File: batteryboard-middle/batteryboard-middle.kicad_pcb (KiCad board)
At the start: 2 copper layers, 45.6 x 45.6 mm, 15 parts, among them J1 FLE-107-01-X-DV-A, J2 FTS-107-01-X-DV-A, J3 Battery Pads, J4 Battery Pads

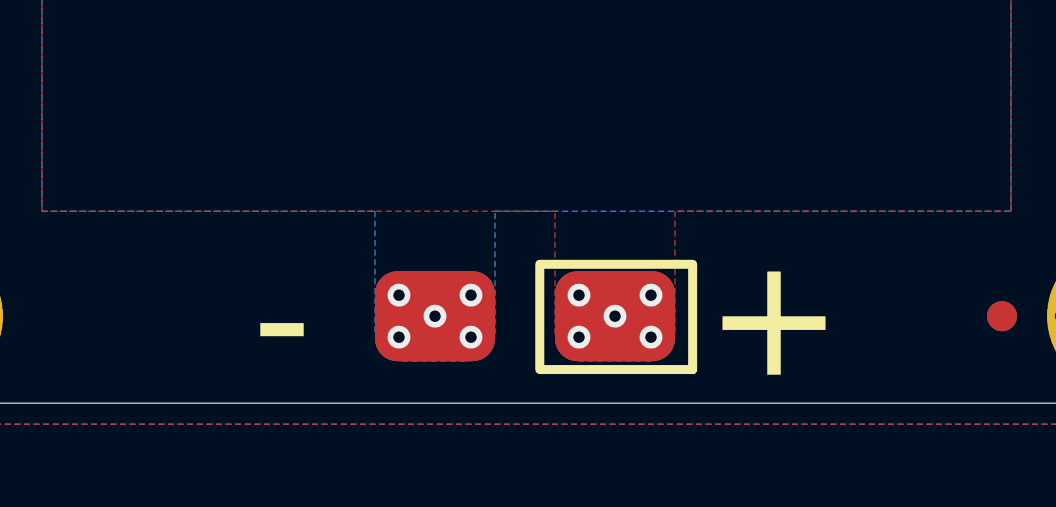
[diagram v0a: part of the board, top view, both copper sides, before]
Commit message: Updated BOMs and STEP files
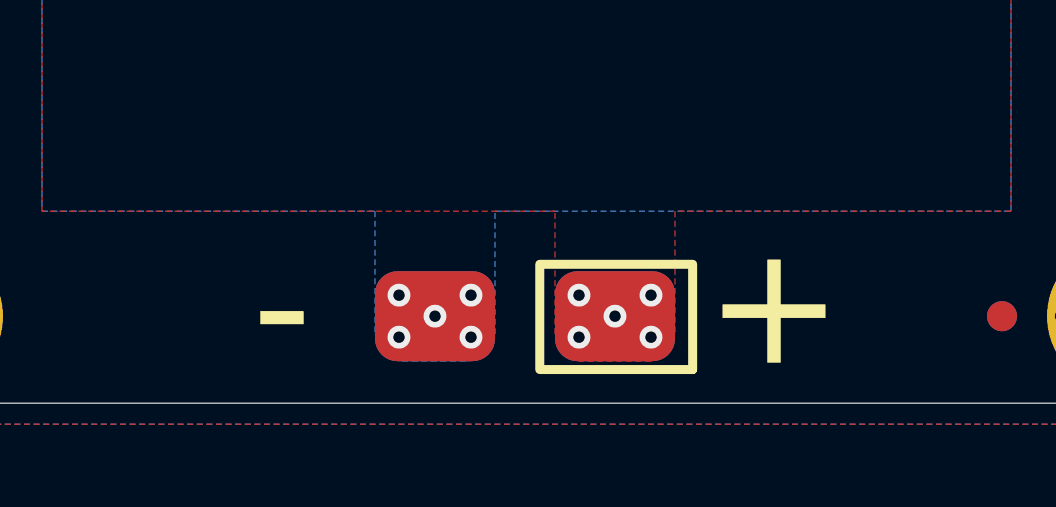
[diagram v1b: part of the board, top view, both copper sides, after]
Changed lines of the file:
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@@
     (property "Sheetfile" "batteryboard-middle.kicad_sch")
     (property "Sheetname" "")
+    (property "exclude_from_bom" "")
     (property "ki_description" "Mounting Hole with connection")
     (property "ki_keywords" "mounting hole")
@@
     (property "Sheetfile" "batteryboard-middle.kicad_sch")
     (property "Sheetname" "")
+    (property "exclude_from_bom" "")
     (property "ki_description" "Mounting Hole with connection")
     (property "ki_keywords" "mounting hole")
@@
     (property "Sheetfile" "batteryboard-middle.kicad_sch")
     (property "Sheetname" "")
+    (property "exclude_from_bom" "")
     (property "ki_description" "Generic connector, single row, 01x02, script generated (kicad-library-utils/schlib/autogen/connector/)")
     (property "ki_keywords" "connector")
-    (attr smd)
+    (attr smd exclude_from_bom)
     (fp_text reference "J3" (at -7.111997 -0.000005 180 unlocked) (layer "F.SilkS") hide
         (effects (font (size 1 1) (thickness 0.15)))
@@
     (descr "Circular Fiducial, 1mm bare copper, 2mm soldermask opening (Level A)")
     (tags "fiducial")
-    (attr smd)
+    (attr smd exclude_from_bom)
     (fp_text reference "REF**" (at 0 -2) (layer "F.SilkS") hide
         (effects (font (size 1 1) (thickness 0.15)))
@@
   (footprint "custom-footprints:pycubed_mini_half" (layer "F.Cu")
     (at 103.9 45)
-    (attr through_hole)
+    (attr through_hole exclude_from_bom)
     (fp_text reference "Ref**" (at 0 0) (layer "F.SilkS") hide
         (effects (font (size 1.27 1.27) (thickness 0.15)))
@@
     (property "Sheetfile" "batteryboard-middle.kicad_sch")
     (property "Sheetname" "")
+    (property "exclude_from_bom" "")
     (property "ki_description" "Mounting Hole with connection")
     (property "ki_keywords" "mounting hole")
@@
     (property "Sheetfile" "batteryboard-middle.kicad_sch")
     (property "Sheetname" "")
+    (property "exclude_from_bom" "")
     (property "ki_description" "Mounting Hole with connection")
     (property "ki_keywords" "mounting hole")
@@
     (descr "Circular Fiducial, 1mm bare copper, 2mm soldermask opening (Level A)")
     (tags "fiducial")
-    (attr smd)
+    (attr smd exclude_from_bom)
     (fp_text reference "REF**" (at 0 -2) (layer "F.SilkS") hide
         (effects (font (size 1 1) (thickness 0.15)))
@@
     (descr "Circular Fiducial, 1mm bare copper, 2mm soldermask opening (Level A)")
     (tags "fiducial")
-    (attr smd)
+    (attr smd exclude_from_bom)
     (fp_text reference "REF**" (at 0 -2) (layer "F.SilkS") hide
         (effects (font (size 1 1) (thickness 0.15)))
@@
     (property "Sheetfile" "batteryboard-middle.kicad_sch")
     (property "Sheetname" "")
+    (property "exclude_from_bom" "")
     (property "ki_description" "Generic connector, single row, 01x02, script generated (kicad-library-utils/schlib/autogen/connector/)")
     (property "ki_keywords" "connector")
-    (attr smd)
+    (attr smd exclude_from_bom)
     (fp_text reference "J4" (at -7.112 0 180 unlocked) (layer "B.SilkS") hide
         (effects (font (size 1 1) (thickness 0.15)) (justify mirror))
@@
     (descr "Circular Fiducial, 1mm bare copper, 2mm soldermask opening (Level A)")
     (tags "fiducial")
-    (attr smd)
+    (attr smd exclude_from_bom)
     (fp_text reference "REF**" (at 0 2) (layer "B.SilkS") hide
         (effects (font (size 1 1) (thickness 0.15)) (justify mirror))
@@
     (descr "Circular Fiducial, 1mm bare copper, 2mm soldermask opening (Level A)")
     (tags "fiducial")
-    (attr smd)
+    (attr smd exclude_from_bom)
     (fp_text reference "REF**" (at 0 2) (layer "B.SilkS") hide
         (effects (font (size 1 1) (thickness 0.15)) (justify mirror))
@@
     (descr "Circular Fiducial, 1mm bare copper, 2mm soldermask opening (Level A)")
     (tags "fiducial")
-    (attr smd)
+    (attr smd exclude_from_bom)
     (fp_text reference "REF**" (at 0 2) (layer "B.SilkS") hide
         (effects (font (size 1 1) (thickness 0.15)) (justify mirror))
@@
   (gr_line (start 123.1 88.3) (end 83.3 88.3)
     (stroke (width 0.0254) (type solid)) (layer "Edge.Cuts"))
-  (gr_text "+" (at 111.5 85.5) (layer "B.SilkS")
+  (gr_text "+" (at 111.5 85.1) (layer "B.SilkS")
     (effects (font (size 4 4) (thickness 0.7)) (justify mirror))
   )
-  (gr_text "-" (at 95.1 85.5) (layer "B.SilkS")
+  (gr_text "-" (at 95.1 85.1) (layer "B.SilkS")
     (effects (font (size 4 4) (thickness 0.7)) (justify mirror))
   )
-  (gr_text "+" (at 111.5 85.5) (layer "F.SilkS")
+  (gr_text "+" (at 111.5 85.1) (layer "F.SilkS")
     (effects (font (size 4 4) (thickness 0.7)) (justify mirror))
   )
-  (gr_text "-" (at 95.1 85.5) (layer "F.SilkS")
+  (gr_text "-" (at 95.1 85.1) (layer "F.SilkS")
     (effects (font (size 4 4) (thickness 0.7)) (justify mirror))
   )
@@
     (effects (font (size 0.635 0.635) (thickness 0.1524)) (justify right))
   )
+  (dimension (type aligned) (layer "Dwgs.User")
+    (pts (xy 80.4 45.6) (xy 126 45.600006))
+    (height -6.729953)
+    (gr_text "1795.2756 mils" (at 103.200001 37.72005 359.9999925) (layer "Dwgs.User")
+      (effects (font (size 1 1) (thickness 0.15)))
+    )
+    (format (prefix "") (suffix "") (units 3) (units_format 1) (precision 4))
+    (style (thickness 0.15) (arrow_length 1.27) (text_position_mode 0) (extension_height 0.58642) (extension_offset 0.5) keep_text_aligned)
+  )
+  (dimension (type aligned) (layer "Dwgs.User")
+    (pts (xy 83.3 42.7) (xy 83.3 88.3))
+    (height 6.9)
+    (gr_text "1795.2756 mils" (at 75.25 65.5 90) (layer "Dwgs.User")
+      (effects (font (size 1 1) (thickness 0.15)))
+    )
+    (format (prefix "") (suffix "") (units 3) (units_format 1) (precision 4))
+    (style (thickness 0.15) (arrow_length 1.27) (text_position_mode 0) (extension_height 0.58642) (extension_offset 0.5) keep_text_aligned)
+  )
   (via (at 86.47 55.92) (size 0.762) (drill 0.381) (layers "F.Cu" "B.Cu") (net 1))
